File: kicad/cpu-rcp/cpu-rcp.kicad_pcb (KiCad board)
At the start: 2 copper layers, 86.4 x 63.5 mm, 79 parts, among them P1 RDRAM-EDGE, P5 NINTENDO-64_PINHEAD-25X2, SW1 Reset, U1 9480F, U10 CPU-NUS, U6 PIF-NUS, U7 MX8330, U9 RCP-NUS, X1 14.318MHz

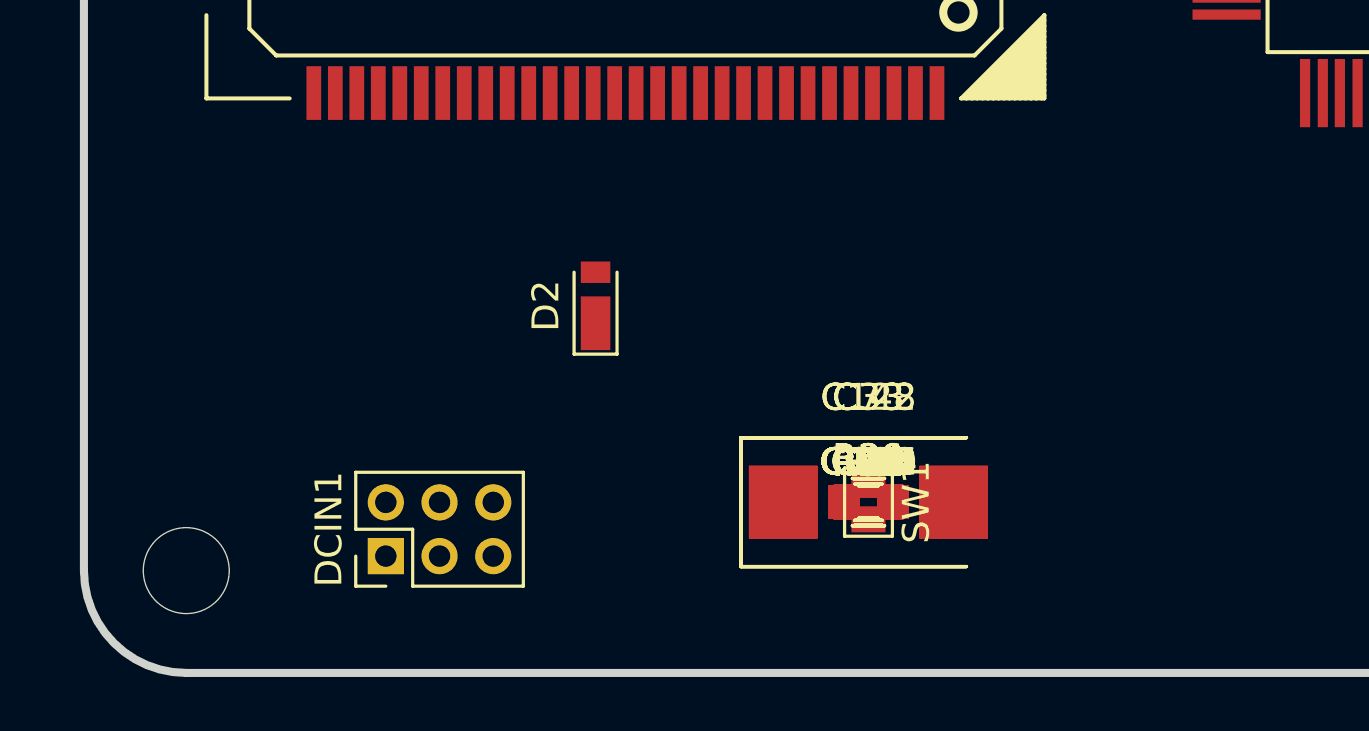
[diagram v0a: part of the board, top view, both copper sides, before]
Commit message: Work in progress, laying around
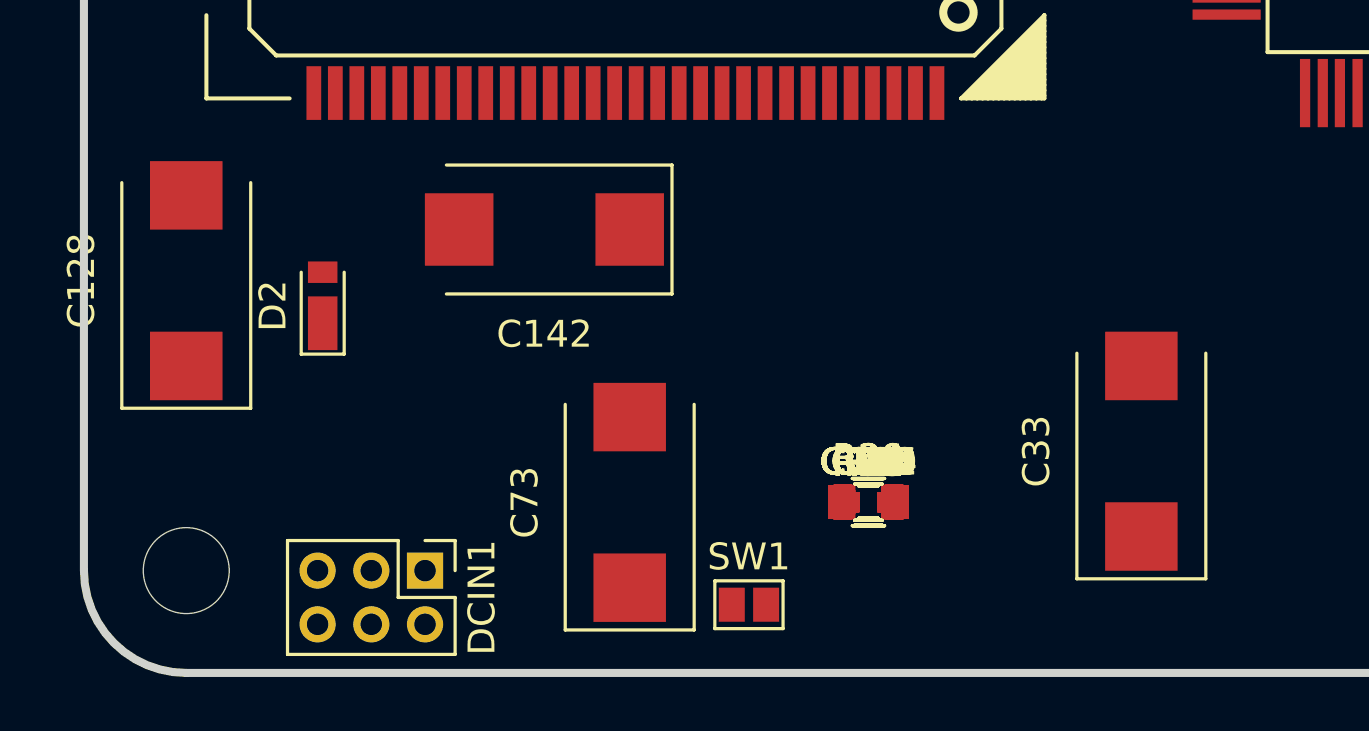
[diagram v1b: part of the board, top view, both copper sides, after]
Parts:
- moved C128 26.7 mm to (29.2, 74.3), turned to 90 degrees
- moved C142 15.8 mm to (42.5, 72.4), turned to 180 degrees
- moved C33 10.3 mm to (64.8, 80.6), turned to 90 degrees
- moved D2 10.2 mm to (34.3, 74.9)
- moved C73 8.89 mm to (45.7, 82.5), turned to 90 degrees
- moved SW1 5.86 mm to (50.2, 86.4), turned to 90 degrees
- moved DCIN1 1.56 mm to (38.1, 85.1), turned to 270 degrees
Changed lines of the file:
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@@
   )
   (module n64:connector-molex-87833-0620 (layer F.Cu)
-    (at 36.64 84.55 90)
+    (at 38.1 85.09 270)
     (descr "Through hole straight pin header, 2x03, 2.00mm pitch, double rows")
     (tags "Through hole pin header THT 2x03 2.00mm double row")
-    (fp_text reference DCIN1 (at 1 -2.12 90) (layer F.SilkS)
+    (fp_text reference DCIN1 (at 1 -2.12 270) (layer F.SilkS)
       (effects (font (size 1 1) (thickness 0.15)))
     )
-    (fp_text value "Power Input" (at 1 6.12 90) (layer F.Fab)
+    (fp_text value "Power Input" (at 1 6.12 270) (layer F.Fab)
       (effects (font (size 1 1) (thickness 0.15)))
     )
@@
     (fp_line (start 3.3 5.3) (end 3.3 -1.3) (layer F.CrtYd) (width 0.05))
     (fp_line (start 3.3 -1.3) (end -1.3 -1.3) (layer F.CrtYd) (width 0.05))
-    (pad 1 thru_hole rect (at 0 0 90) (size 1.35 1.35) (drill 0.8) (layers *.Cu *.Mask)
+    (pad 1 thru_hole rect (at 0 0 270) (size 1.35 1.35) (drill 0.8) (layers *.Cu *.Mask)
       (net 6 GND))
-    (pad 2 thru_hole oval (at 2 0 90) (size 1.35 1.35) (drill 0.8) (layers *.Cu *.Mask)
+    (pad 2 thru_hole oval (at 2 0 270) (size 1.35 1.35) (drill 0.8) (layers *.Cu *.Mask)
       (net 6 GND))
-    (pad 3 thru_hole oval (at 0 2 90) (size 1.35 1.35) (drill 0.8) (layers *.Cu *.Mask)
+    (pad 3 thru_hole oval (at 0 2 270) (size 1.35 1.35) (drill 0.8) (layers *.Cu *.Mask)
       (net 10 VTERM))
-    (pad 4 thru_hole oval (at 2 2 90) (size 1.35 1.35) (drill 0.8) (layers *.Cu *.Mask)
+    (pad 4 thru_hole oval (at 2 2 270) (size 1.35 1.35) (drill 0.8) (layers *.Cu *.Mask)
       (net 105 ENABLE))
-    (pad 5 thru_hole oval (at 0 4 90) (size 1.35 1.35) (drill 0.8) (layers *.Cu *.Mask)
+    (pad 5 thru_hole oval (at 0 4 270) (size 1.35 1.35) (drill 0.8) (layers *.Cu *.Mask)
       (net 56 +3V3))
-    (pad 6 thru_hole oval (at 2 4 90) (size 1.35 1.35) (drill 0.8) (layers *.Cu *.Mask)
+    (pad 6 thru_hole oval (at 2 4 270) (size 1.35 1.35) (drill 0.8) (layers *.Cu *.Mask)
       (net 56 +3V3))
     (model ${KIPRJMOD}/../packages3d/molex-87833-0620.wrl
@@
     (pad 28 smd rect (at -8.890063 5.579938 270) (size 0.7 1.6) (layers B.Cu B.Paste B.Mask)
       (net 56 +3V3))
-    (model ${KIPRJMOD}/../packages3d/SOIC-28W_7.5x17.9mm_Pitch1.27mm.wrl
+    (model ${KIPRJMOD}/../packages3d/SOIC-28_7.5x17.9mm_Pitch1.27mm.wrl
       (at (xyz -0.025 0 0))
       (scale (xyz 1 1 1))
@@
   )
   (module n64:CP_Tantalum_Case-D_EIA-7343-31_Reflow (layer F.Cu)
-    (at 54.61 82.540001)
+    (at 64.77 80.645 90)
     (descr "Tantalum capacitor, Case D, EIA 7343-31, 7.3x4.3x2.8mm, Reflow soldering footprint")
     (tags "capacitor tantalum smd")
     (attr smd)
-    (fp_text reference C33 (at 0 -3.9) (layer F.SilkS)
+    (fp_text reference C33 (at 0 -3.9 90) (layer F.SilkS)
       (effects (font (size 1 1) (thickness 0.15)))
     )
-    (fp_text value 68uF (at 0 3.9) (layer F.Fab)
+    (fp_text value 68uF (at 0 3.9 90) (layer F.Fab)
       (effects (font (size 1 1) (thickness 0.15)))
     )
@@
     (fp_line (start -4.75 2.4) (end 3.65 2.4) (layer F.SilkS) (width 0.12))
     (fp_line (start -4.75 -2.4) (end -4.75 2.4) (layer F.SilkS) (width 0.12))
-    (pad 1 smd rect (at -3.175 0) (size 2.55 2.7) (layers F.Cu F.Paste F.Mask)
+    (pad 1 smd rect (at -3.175 0 90) (size 2.55 2.7) (layers F.Cu F.Paste F.Mask)
       (net 57 "Net-(C33-Pad1)"))
-    (pad 2 smd rect (at 3.175 0) (size 2.55 2.7) (layers F.Cu F.Paste F.Mask)
+    (pad 2 smd rect (at 3.175 0 90) (size 2.55 2.7) (layers F.Cu F.Paste F.Mask)
       (net 6 GND))
     (model Capacitors_Tantalum_SMD.3dshapes/CP_Tantalum_Case-D_EIA-7343-31.wrl
@@
   )
   (module n64:CP_Tantalum_Case-D_EIA-7343-31_Reflow (layer F.Cu)
-    (at 54.61 82.540001)
+    (at 45.72 82.55 90)
     (descr "Tantalum capacitor, Case D, EIA 7343-31, 7.3x4.3x2.8mm, Reflow soldering footprint")
     (tags "capacitor tantalum smd")
     (attr smd)
-    (fp_text reference C73 (at 0 -3.9) (layer F.SilkS)
+    (fp_text reference C73 (at 0 -3.9 90) (layer F.SilkS)
       (effects (font (size 1 1) (thickness 0.15)))
     )
-    (fp_text value 68uF (at 0 3.9) (layer F.Fab)
+    (fp_text value 68uF (at 0 3.9 90) (layer F.Fab)
       (effects (font (size 1 1) (thickness 0.15)))
     )
@@
     (fp_line (start -4.75 2.4) (end 3.65 2.4) (layer F.SilkS) (width 0.12))
     (fp_line (start -4.75 -2.4) (end -4.75 2.4) (layer F.SilkS) (width 0.12))
-    (pad 1 smd rect (at -3.175 0) (size 2.55 2.7) (layers F.Cu F.Paste F.Mask)
+    (pad 1 smd rect (at -3.175 0 90) (size 2.55 2.7) (layers F.Cu F.Paste F.Mask)
       (net 10 VTERM))
-    (pad 2 smd rect (at 3.175 0) (size 2.55 2.7) (layers F.Cu F.Paste F.Mask)
+    (pad 2 smd rect (at 3.175 0 90) (size 2.55 2.7) (layers F.Cu F.Paste F.Mask)
       (net 6 GND))
     (model Capacitors_Tantalum_SMD.3dshapes/CP_Tantalum_Case-D_EIA-7343-31.wrl
@@
   )
   (module n64:CP_Tantalum_Case-D_EIA-7343-31_Reflow (layer F.Cu)
-    (at 54.61 82.540001)
+    (at 29.21 74.295 90)
     (descr "Tantalum capacitor, Case D, EIA 7343-31, 7.3x4.3x2.8mm, Reflow soldering footprint")
     (tags "capacitor tantalum smd")
     (attr smd)
-    (fp_text reference C128 (at 0 -3.9) (layer F.SilkS)
+    (fp_text reference C128 (at 0 -3.9 90) (layer F.SilkS)
       (effects (font (size 1 1) (thickness 0.15)))
     )
-    (fp_text value 10uF (at 0 3.9) (layer F.Fab)
+    (fp_text value 10uF (at 0 3.9 90) (layer F.Fab)
       (effects (font (size 1 1) (thickness 0.15)))
     )
@@
     (fp_line (start -4.75 2.4) (end 3.65 2.4) (layer F.SilkS) (width 0.12))
     (fp_line (start -4.75 -2.4) (end -4.75 2.4) (layer F.SilkS) (width 0.12))
-    (pad 1 smd rect (at -3.175 0) (size 2.55 2.7) (layers F.Cu F.Paste F.Mask)
+    (pad 1 smd rect (at -3.175 0 90) (size 2.55 2.7) (layers F.Cu F.Paste F.Mask)
       (net 103 "Net-(C128-Pad1)"))
-    (pad 2 smd rect (at 3.175 0) (size 2.55 2.7) (layers F.Cu F.Paste F.Mask)
+    (pad 2 smd rect (at 3.175 0 90) (size 2.55 2.7) (layers F.Cu F.Paste F.Mask)
       (net 6 GND))
     (model Capacitors_Tantalum_SMD.3dshapes/CP_Tantalum_Case-D_EIA-7343-31.wrl
@@
   )
   (module n64:CP_Tantalum_Case-D_EIA-7343-31_Reflow (layer F.Cu)
-    (at 54.61 82.540001)
+    (at 42.545 72.39 180)
     (descr "Tantalum capacitor, Case D, EIA 7343-31, 7.3x4.3x2.8mm, Reflow soldering footprint")
     (tags "capacitor tantalum smd")
     (attr smd)
-    (fp_text reference C142 (at 0 -3.9) (layer F.SilkS)
+    (fp_text reference C142 (at 0 -3.9 180) (layer F.SilkS)
       (effects (font (size 1 1) (thickness 0.15)))
     )
-    (fp_text value 33uF (at 0 3.9) (layer F.Fab)
+    (fp_text value 33uF (at 0 3.9 180) (layer F.Fab)
       (effects (font (size 1 1) (thickness 0.15)))
     )
@@
     (fp_line (start -4.75 2.4) (end 3.65 2.4) (layer F.SilkS) (width 0.12))
     (fp_line (start -4.75 -2.4) (end -4.75 2.4) (layer F.SilkS) (width 0.12))
-    (pad 1 smd rect (at -3.175 0) (size 2.55 2.7) (layers F.Cu F.Paste F.Mask)
+    (pad 1 smd rect (at -3.175 0 180) (size 2.55 2.7) (layers F.Cu F.Paste F.Mask)
       (net 56 +3V3))
-    (pad 2 smd rect (at 3.175 0) (size 2.55 2.7) (layers F.Cu F.Paste F.Mask)
+    (pad 2 smd rect (at 3.175 0 180) (size 2.55 2.7) (layers F.Cu F.Paste F.Mask)
       (net 6 GND))
     (model Capacitors_Tantalum_SMD.3dshapes/CP_Tantalum_Case-D_EIA-7343-31.wrl
@@
   )
   (module n64:D_TUMD2 (layer F.Cu)
-    (at 44.45 74.93 90)
+    (at 34.29 74.93 90)
     (descr "ROHM - TUMD2")
     (tags TUMD2)
@@
   )
   (module n64:Connectors_GS2 (layer F.Cu)
-    (at 54.61 82.540001)
+    (at 50.16 86.36 90)
     (descr "2-pin solder bridge")
     (tags "solder bridge")
     (attr smd)
-    (fp_text reference SW1 (at 1.78 0 90) (layer F.SilkS)
+    (fp_text reference SW1 (at 1.78 0 180) (layer F.SilkS)
       (effects (font (size 1 1) (thickness 0.15)))
     )
-    (fp_text value Reset (at -1.8 0 90) (layer F.Fab)
+    (fp_text value Reset (at -1.8 0 180) (layer F.Fab)
       (effects (font (size 1 1) (thickness 0.15)))
     )
@@
     (fp_line (start 0.89 1.27) (end -0.89 1.27) (layer F.SilkS) (width 0.12))
     (fp_line (start -0.89 -1.27) (end 0.89 -1.27) (layer F.SilkS) (width 0.12))
-    (pad 1 smd rect (at 0 -0.64) (size 1.27 0.97) (layers F.Cu F.Paste F.Mask)
+    (pad 1 smd rect (at 0 -0.64 90) (size 1.27 0.97) (layers F.Cu F.Paste F.Mask)
       (net 101 "Net-(C123-Pad1)"))
-    (pad 2 smd rect (at 0 0.64) (size 1.27 0.97) (layers F.Cu F.Paste F.Mask)
+    (pad 2 smd rect (at 0 0.64 90) (size 1.27 0.97) (layers F.Cu F.Paste F.Mask)
       (net 6 GND))
   )
